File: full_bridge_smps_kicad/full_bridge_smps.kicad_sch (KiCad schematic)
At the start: 0 parts

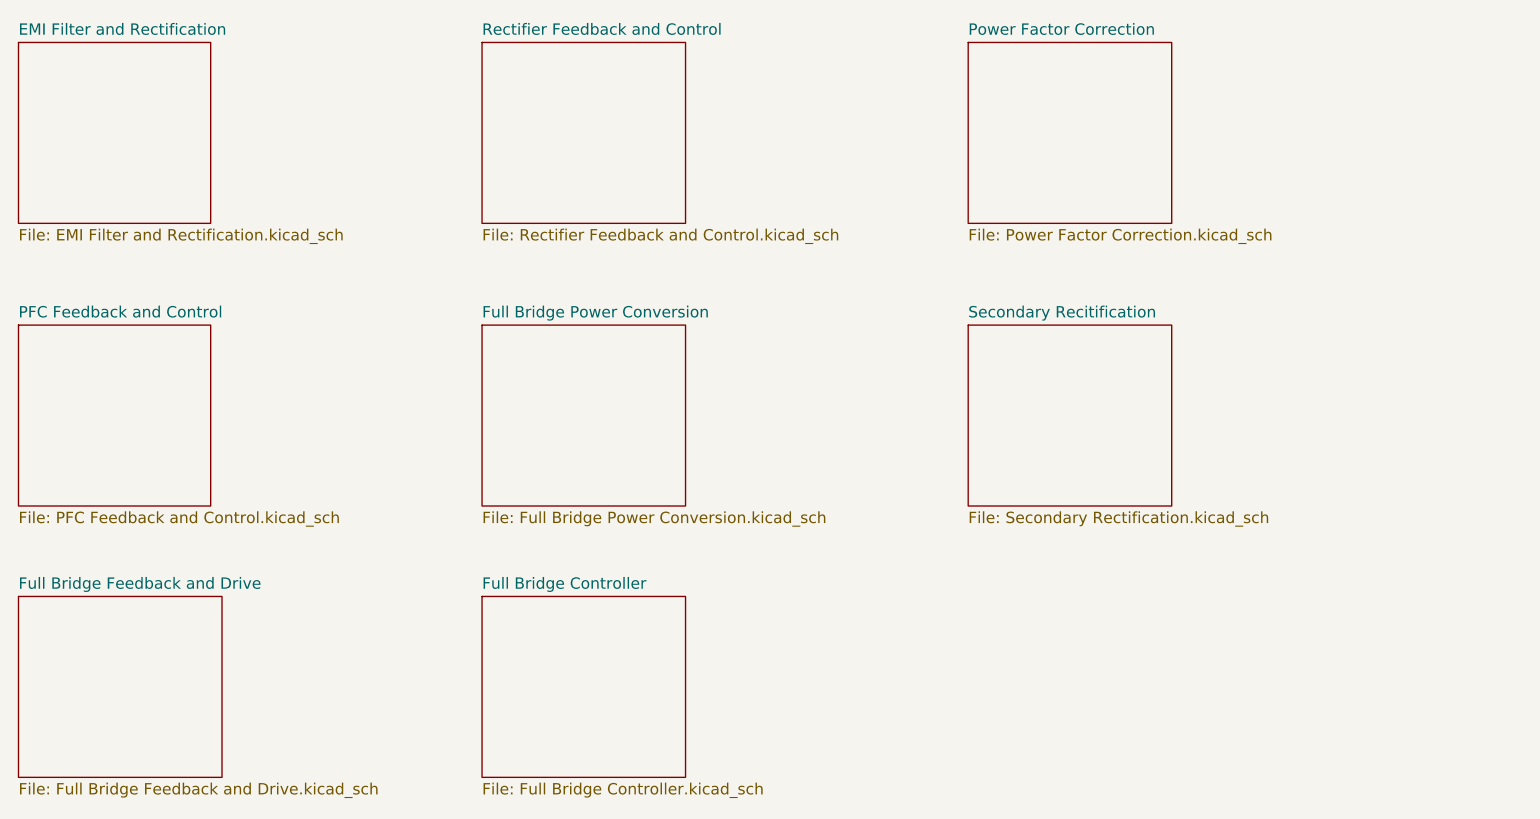
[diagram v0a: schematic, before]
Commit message: A bit of refactoring, saving work for the day
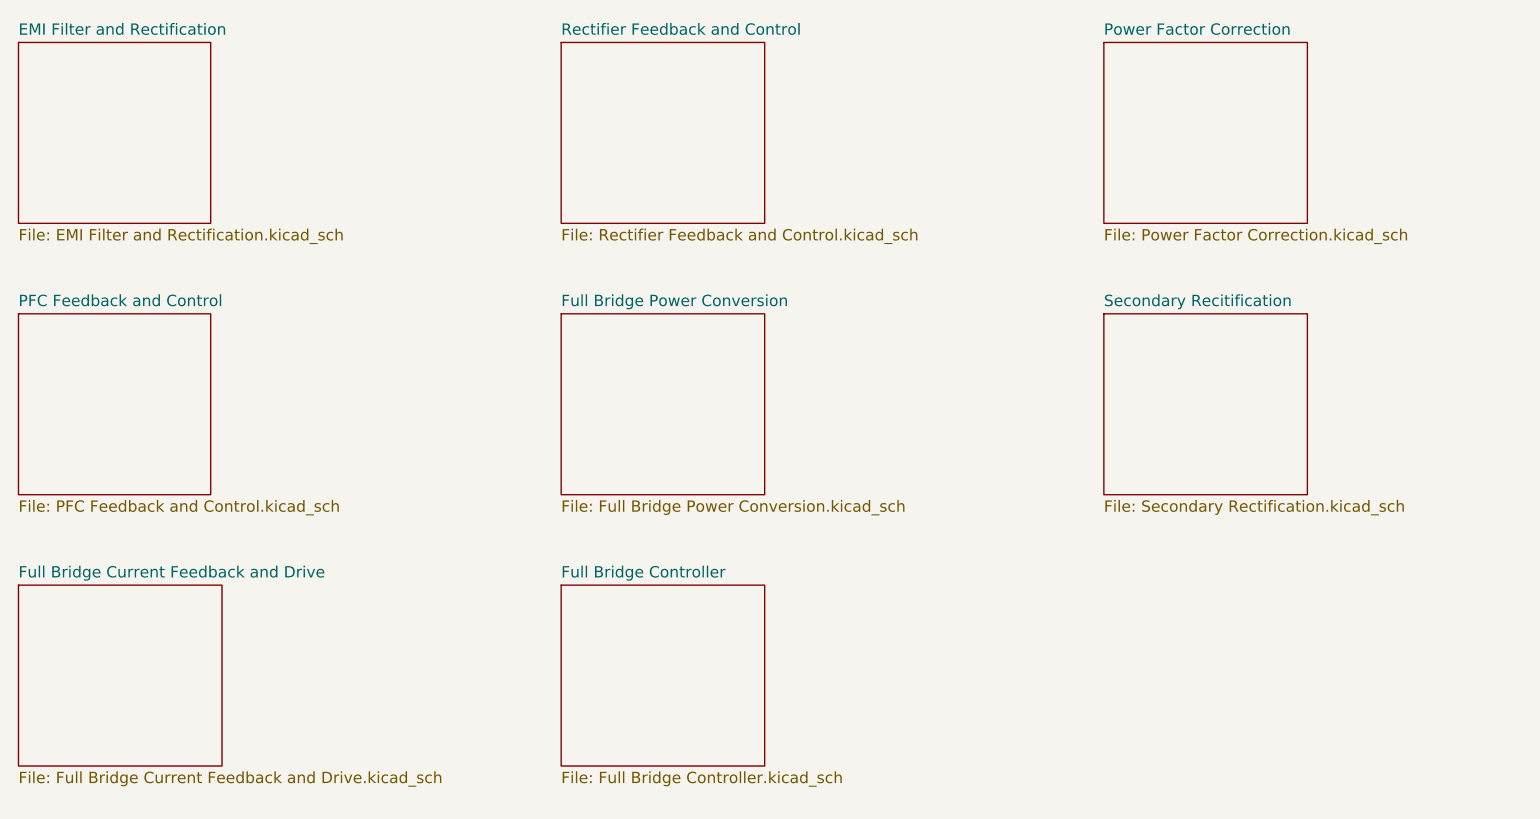
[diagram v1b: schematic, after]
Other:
- removed sheet Full Bridge Feedback and Drive
- added sheet Full Bridge Current Feedback and Drive (Full Bridge Current Feedback and Drive.kicad_sch)
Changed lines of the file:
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@@
     (rev "1.0.0")
+  )
+  (sheet (at 24.13 77.47) (size 22.86 20.32) (fields_autoplaced)
+    (stroke (width 0.1524) (type solid))
+    (fill (color 0 0 0 0.0000))
+    (property "Sheetname" "Full Bridge Current Feedback and Drive" (at 24.13 76.7584 0)
+      (effects (font (size 1.27 1.27)) (justify left bottom))
+    )
+    (property "Sheetfile" "Full Bridge Current Feedback and Drive.kicad_sch" (at 24.13 98.3746 0)
+      (effects (font (size 1.27 1.27)) (justify left top))
+    )
+    (instances
+      (project "full_bridge_smps"
+        (path "/f89200e7-8fc9-4acb-bb2b-7da3a53d52f5" (page "8"))
+      )
+    )
   )
   (sheet (at 24.13 16.51) (size 21.59 20.32) (fields_autoplaced)
@@
     )
   )
-  (sheet (at 24.13 78.74) (size 22.86 20.32) (fields_autoplaced)
+  (sheet (at 85.09 46.99) (size 22.86 20.32) (fields_autoplaced)
     (stroke (width 0.1524) (type solid))
     (fill (color 0 0 0 0.0000))
-    (property "Sheetname" "Full Bridge Feedback and Drive" (at 24.13 78.0284 0)
+    (property "Sheetname" "Full Bridge Power Conversion" (at 85.09 46.2784 0)
       (effects (font (size 1.27 1.27)) (justify left bottom))
     )
-    (property "Sheetfile" "Full Bridge Feedback and Drive.kicad_sch" (at 24.13 99.6446 0)
-      (effects (font (size 1.27 1.27)) (justify left top))
-    )
-    (instances
-      (project "full_bridge_smps"
-        (path "/f89200e7-8fc9-4acb-bb2b-7da3a53d52f5" (page "8"))
-      )
-    )
-  )
-  (sheet (at 76.2 48.26) (size 22.86 20.32) (fields_autoplaced)
-    (stroke (width 0.1524) (type solid))
-    (fill (color 0 0 0 0.0000))
-    (property "Sheetname" "Full Bridge Power Conversion" (at 76.2 47.5484 0)
-      (effects (font (size 1.27 1.27)) (justify left bottom))
-    )
-    (property "Sheetfile" "Full Bridge Power Conversion.kicad_sch" (at 76.2 69.1646 0)
+    (property "Sheetfile" "Full Bridge Power Conversion.kicad_sch" (at 85.09 67.8946 0)
       (effects (font (size 1.27 1.27)) (justify left top))
     )
@@
     )
   )
-  (sheet (at 76.2 78.74) (size 22.86 20.32) (fields_autoplaced)
+  (sheet (at 85.09 77.47) (size 22.86 20.32) (fields_autoplaced)
     (stroke (width 0.1524) (type solid))
     (fill (color 0 0 0 0.0000))
-    (property "Sheetname" "Full Bridge Controller" (at 76.2 78.0284 0)
+    (property "Sheetname" "Full Bridge Controller" (at 85.09 76.7584 0)
       (effects (font (size 1.27 1.27)) (justify left bottom))
     )
-    (property "Sheetfile" "Full Bridge Controller.kicad_sch" (at 76.2 99.6446 0)
+    (property "Sheetfile" "Full Bridge Controller.kicad_sch" (at 85.09 98.3746 0)
       (effects (font (size 1.27 1.27)) (justify left top))
     )
@@
     )
   )
-  (sheet (at 130.81 48.26) (size 22.86 20.32) (fields_autoplaced)
+  (sheet (at 146.05 46.99) (size 22.86 20.32) (fields_autoplaced)
     (stroke (width 0.1524) (type solid))
     (fill (color 0 0 0 0.0000))
-    (property "Sheetname" "Secondary Recitification" (at 130.81 47.5484 0)
+    (property "Sheetname" "Secondary Recitification" (at 146.05 46.2784 0)
       (effects (font (size 1.27 1.27)) (justify left bottom))
     )
-    (property "Sheetfile" "Secondary Rectification.kicad_sch" (at 130.81 69.1646 0)
+    (property "Sheetfile" "Secondary Rectification.kicad_sch" (at 146.05 67.8946 0)
       (effects (font (size 1.27 1.27)) (justify left top))
     )
@@
     )
   )
-  (sheet (at 130.81 16.51) (size 22.86 20.32) (fields_autoplaced)
+  (sheet (at 146.05 16.51) (size 22.86 20.32) (fields_autoplaced)
     (stroke (width 0.1524) (type solid))
     (fill (color 0 0 0 0.0000))
-    (property "Sheetname" "Power Factor Correction" (at 130.81 15.7984 0)
+    (property "Sheetname" "Power Factor Correction" (at 146.05 15.7984 0)
       (effects (font (size 1.27 1.27)) (justify left bottom))
     )
-    (property "Sheetfile" "Power Factor Correction.kicad_sch" (at 130.81 37.4146 0)
+    (property "Sheetfile" "Power Factor Correction.kicad_sch" (at 146.05 37.4146 0)
       (effects (font (size 1.27 1.27)) (justify left top))
     )
@@
     )
   )
-  (sheet (at 76.2 16.51) (size 22.86 20.32) (fields_autoplaced)
+  (sheet (at 85.09 16.51) (size 22.86 20.32) (fields_autoplaced)
     (stroke (width 0.1524) (type solid))
     (fill (color 0 0 0 0.0000))
-    (property "Sheetname" "Rectifier Feedback and Control" (at 76.2 15.7984 0)
+    (property "Sheetname" "Rectifier Feedback and Control" (at 85.09 15.7984 0)
       (effects (font (size 1.27 1.27)) (justify left bottom))
     )
-    (property "Sheetfile" "Rectifier Feedback and Control.kicad_sch" (at 76.2 37.4146 0)
+    (property "Sheetfile" "Rectifier Feedback and Control.kicad_sch" (at 85.09 37.4146 0)
       (effects (font (size 1.27 1.27)) (justify left top))
     )
@@
     )
   )
-  (sheet (at 24.13 48.26) (size 21.59 20.32) (fields_autoplaced)
+  (sheet (at 24.13 46.99) (size 21.59 20.32) (fields_autoplaced)
     (stroke (width 0.1524) (type solid))
     (fill (color 0 0 0 0.0000))
-    (property "Sheetname" "PFC Feedback and Control" (at 24.13 47.5484 0)
+    (property "Sheetname" "PFC Feedback and Control" (at 24.13 46.2784 0)
       (effects (font (size 1.27 1.27)) (justify left bottom))
     )
-    (property "Sheetfile" "PFC Feedback and Control.kicad_sch" (at 24.13 69.1646 0)
+    (property "Sheetfile" "PFC Feedback and Control.kicad_sch" (at 24.13 67.8946 0)
       (effects (font (size 1.27 1.27)) (justify left top))
     )
